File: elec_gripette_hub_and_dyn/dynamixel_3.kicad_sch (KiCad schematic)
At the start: 27 parts, among them J4 Dynamixel-3, J5 Dynamixel-3, J9 Dynamixel-3, Q1 MMBT3906, U3 CH343P, U4 SN74LVC1G125DBV, U5 SN74LVC1G126DBVR

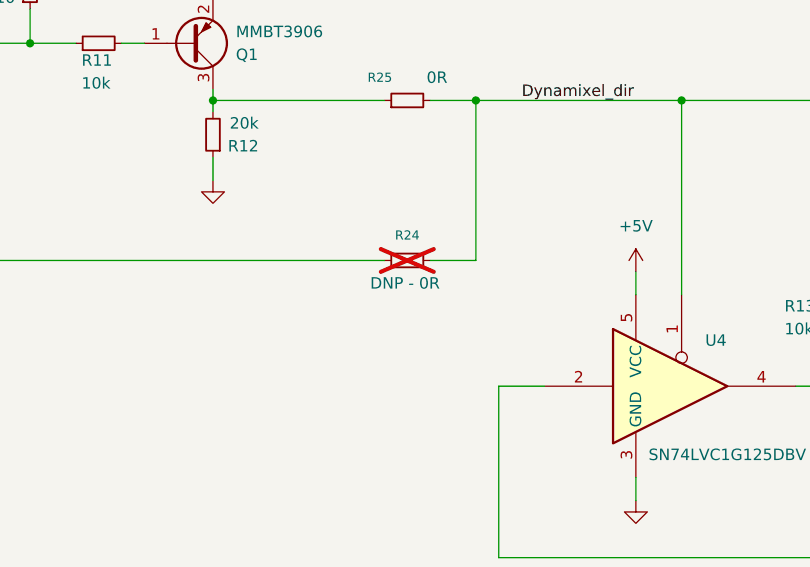
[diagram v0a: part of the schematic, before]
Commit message: [update] Before review
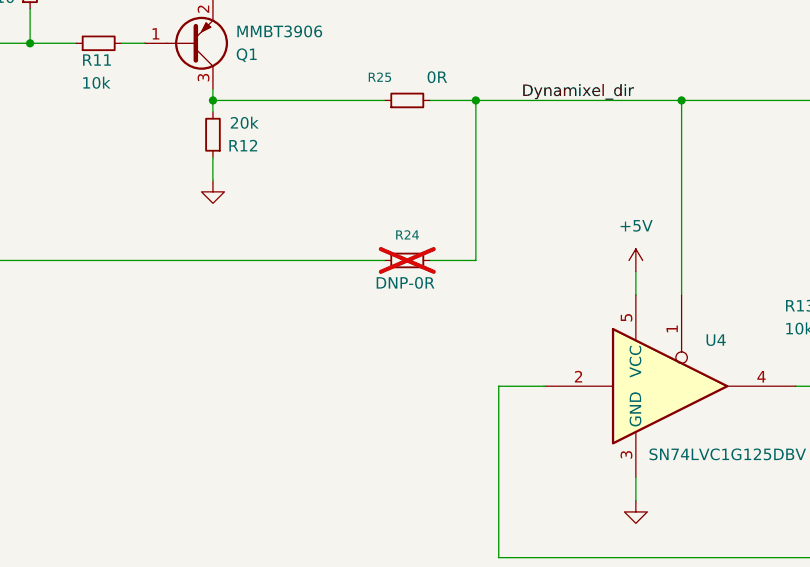
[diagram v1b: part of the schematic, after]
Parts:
- R24: value DNP - 0R -> DNP-0R; footprint Resistor_SMD:R_0402_1005Metric -> Resistor_SMD:R_0603_1608Metric; LCSC Part C17168 -> (none)
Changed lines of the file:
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@@
 			)
 		)
-		(property "Value" "DNP - 0R"
+		(property "Value" "DNP-0R"
 			(at 185.166 109.22 90)
 			(effects
@@
 			)
 		)
-		(property "Footprint" "Resistor_SMD:R_0402_1005Metric"
+		(property "Footprint" "Resistor_SMD:R_0603_1608Metric"
 			(at 185.42 106.68 0)
 			(effects
@@
 			)
 		)
-		(property "LCSC Part" "C17168"
+		(property "LCSC Part" ""
 			(at 185.42 106.68 90)
 			(effects

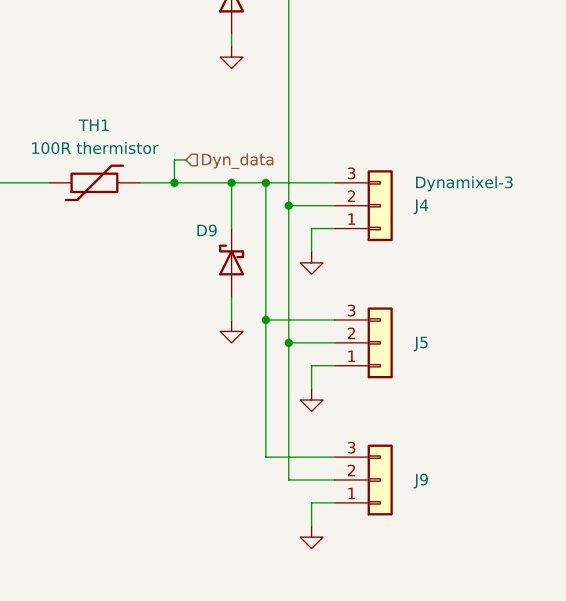
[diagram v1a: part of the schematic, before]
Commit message: [update] gripette + bulkhead -B1 in production @JLCPCB
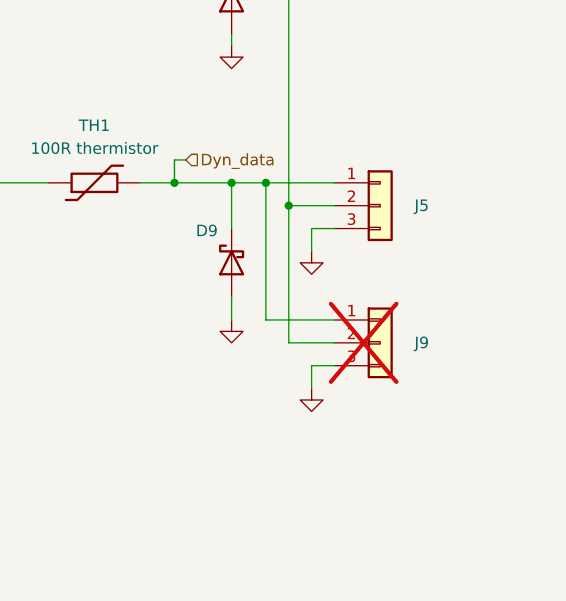
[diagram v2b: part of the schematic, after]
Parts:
- removed J4: Dynamixel-3, Connector_JST:JST_EH_B3B-EH-A_1x03_P2.50mm_Vertical, symbol Connector_Generic:Conn_01x03
- J5: value Dynamixel-3 -> Feetech; footprint Connector_JST:JST_EH_B3B-EH-A_1x03_P2.50mm_Vertical -> Connector_Molex:Molex_SPOX_5267-03A_1x03_P2.50mm_Vertical; FT Rotation Offset (none) -> 180; LCSC Part C160259 -> C293315; Man. JST -> (none); Man. Ref. B3B-EH-A(LF)(SN) -> (none)
- J9: value Dynamixel-3 -> Feetech; footprint Connector_JST:JST_EH_B3B-EH-A_1x03_P2.50mm_Vertical -> Connector_Molex:Molex_SPOX_5267-03A_1x03_P2.50mm_Vertical; FT Rotation Offset (none) -> 180; LCSC Part C160259 -> (none); Man. JST -> (none); Man. Ref. B3B-EH-A(LF)(SN) -> (none); now not fitted
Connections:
- net Dyn_data: now also J5.1 (Pin_1), J9.1 (Pin_1); no longer J5.3 (Pin_3), J9.3 (Pin_3)
- net GND: now also J5.3 (Pin_3), J9.3 (Pin_3); no longer J5.1 (Pin_1), J9.1 (Pin_1)
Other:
- moved on the sheet: J5
